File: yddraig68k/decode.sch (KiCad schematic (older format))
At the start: 31 parts, among them J401 NMI Reset, J402 Ext RUN LED, J403 Conn_01x06, Q401 2N4403, Q402 2N4403, Q403 2N4403, U401 74HC164, U402 74LS08, U403 74LS148, U404 XC95108PC84, X401 40MHz

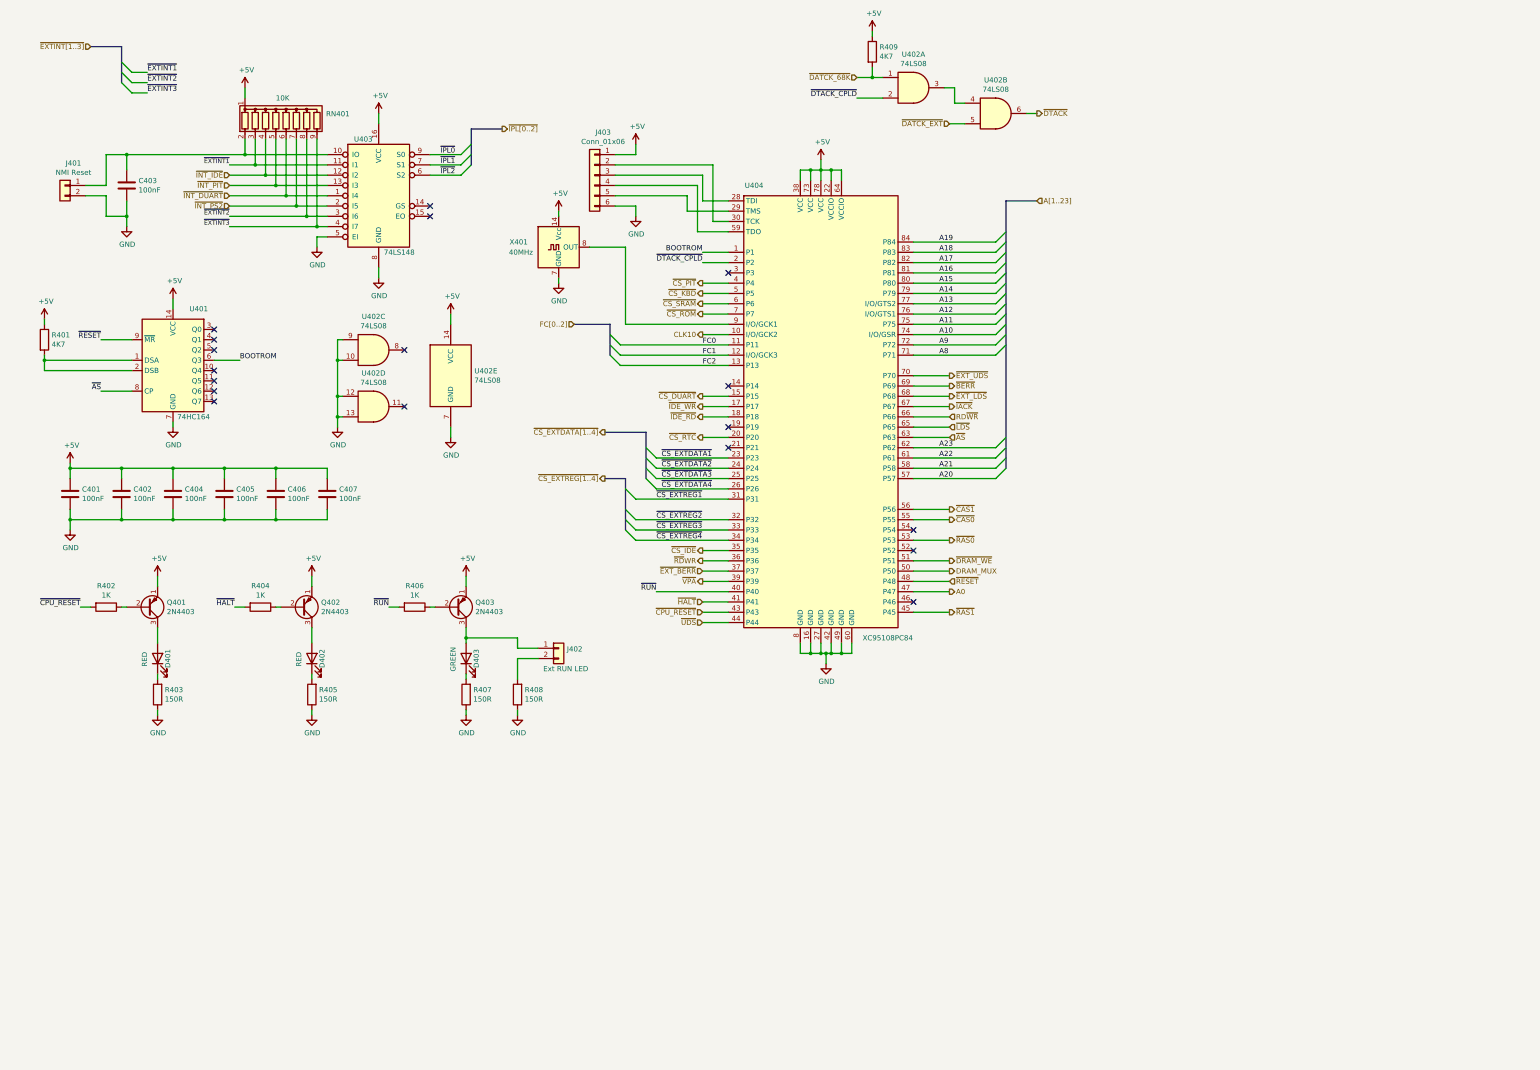
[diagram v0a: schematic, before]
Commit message: Starting changes
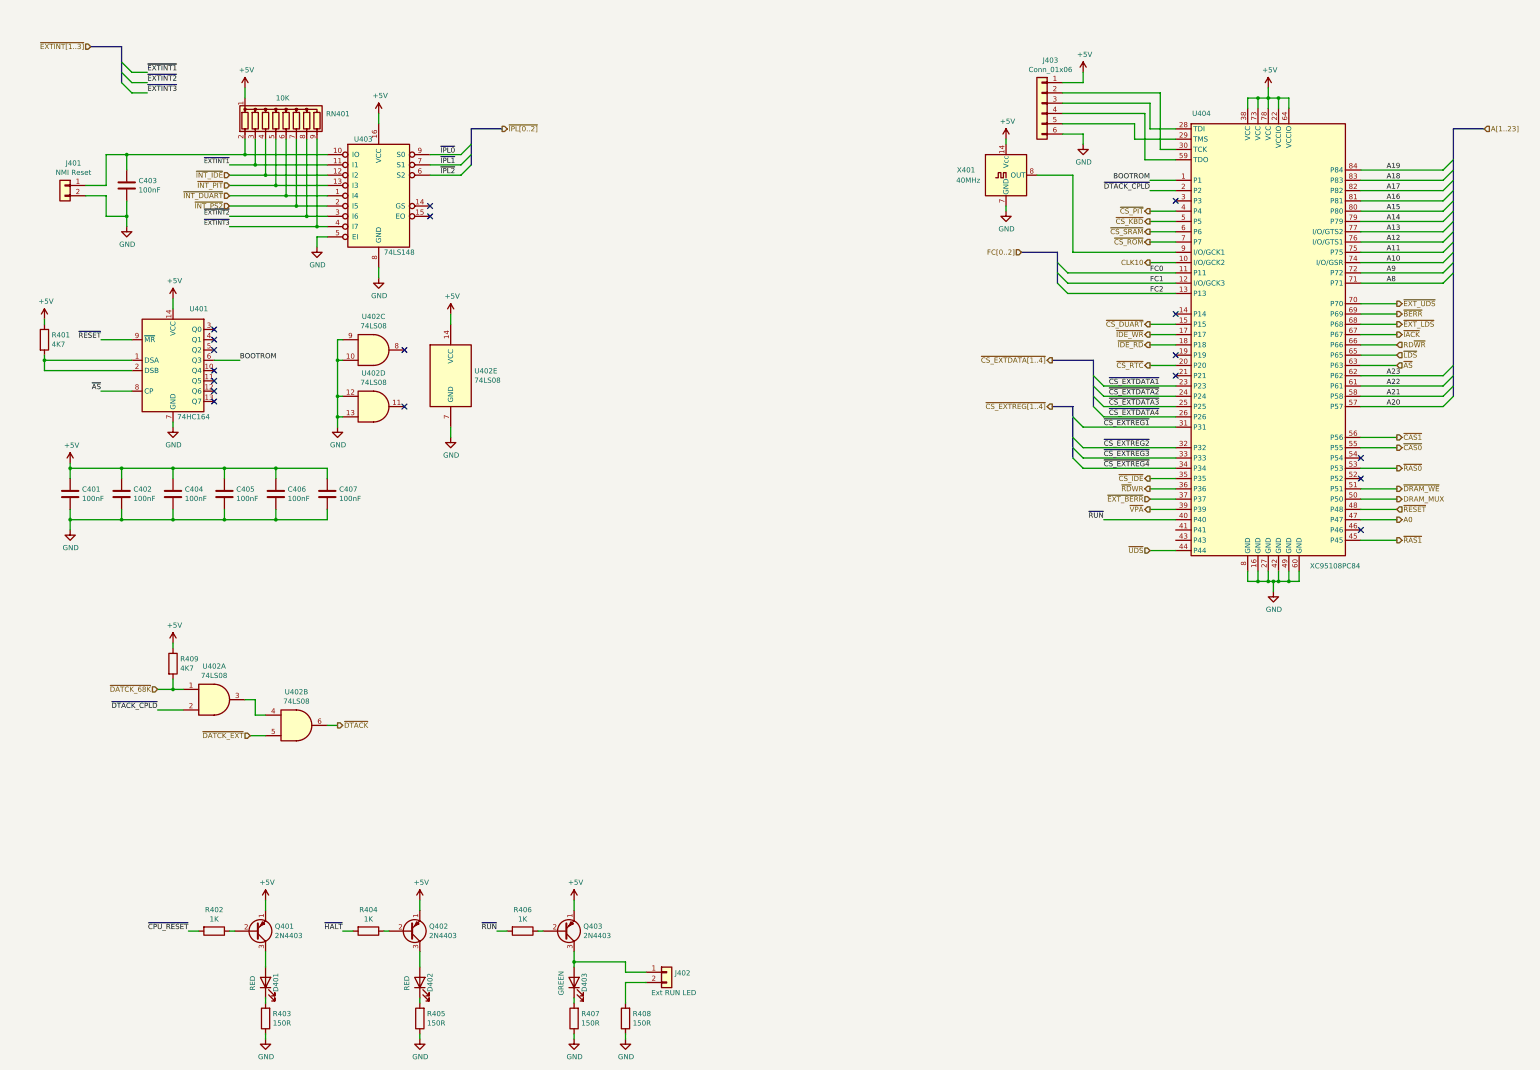
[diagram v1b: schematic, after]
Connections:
- net ~CPU_RESET: no longer U404.43 (P43)
- net ~HALT: no longer U404.41 (P41)
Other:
- moved on the sheet: D401, D402, D403, J402, J403, Q401, Q402, Q403, R402, R403, R404, R405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
